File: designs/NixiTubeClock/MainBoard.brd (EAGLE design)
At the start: 94 x 45 mm, 18 parts, among them IC1 LD117ADT-TR, J1 S2B-PH-SM4, J2 S2B-PH-SM4, J3 S2B-PH-SM4, J4 S2B-PH-SM4, J5 S2B-PH-SM4, J6 S2B-PH-SM4, J7 S2B-PH-SM4

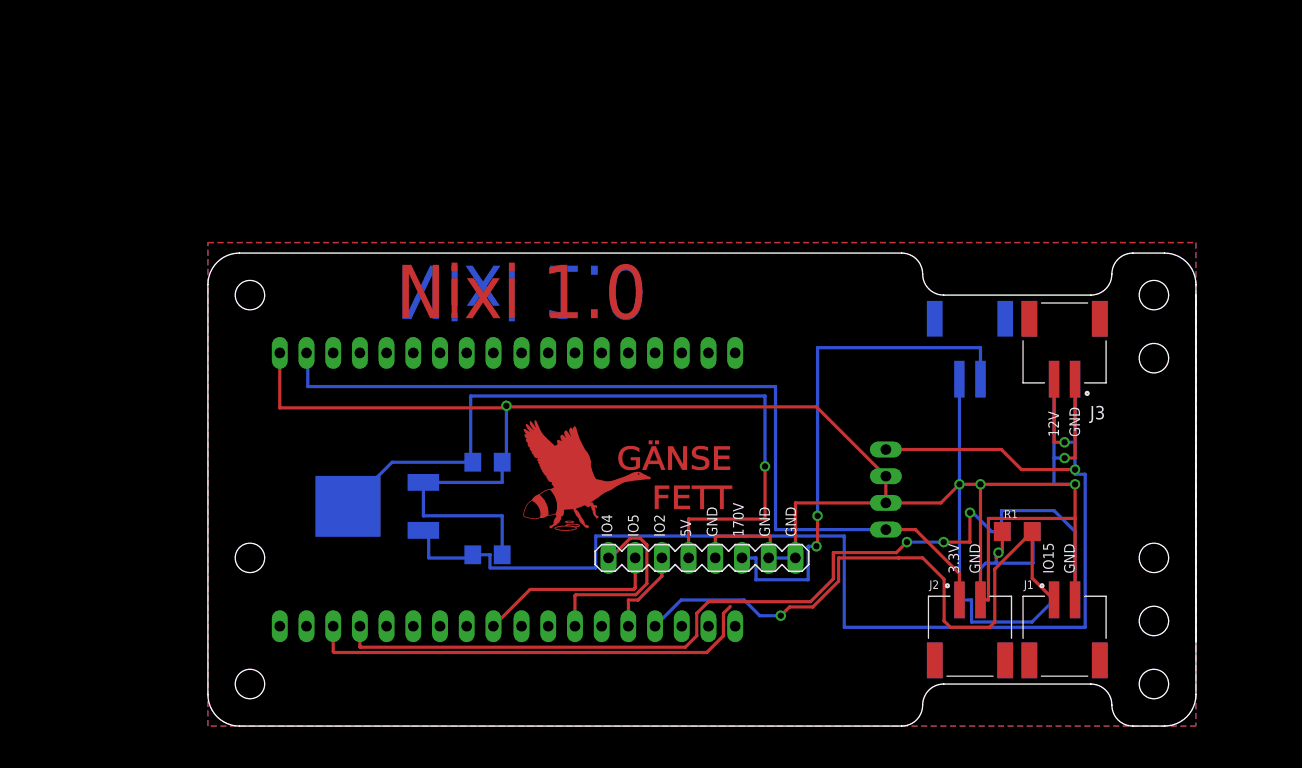
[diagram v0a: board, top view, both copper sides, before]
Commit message: started work on mainboard
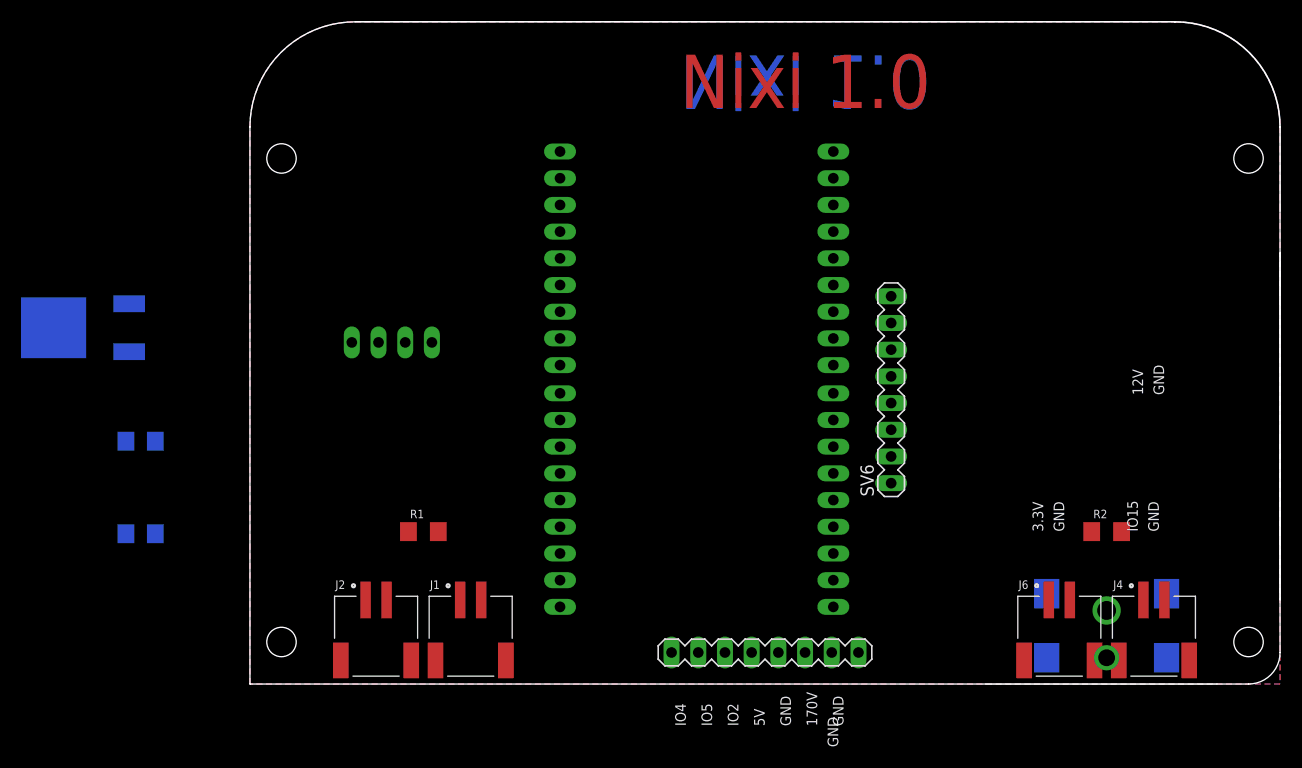
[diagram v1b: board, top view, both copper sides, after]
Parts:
- removed J3, J7: S2B-PH-SM4, CommonParts:JST_S2B-PH-SM4-TB(LF)(SN)
- added SV6: (no value), CommonParts:MA08-1
- J5: value S2B-PH-SM4 -> PJ-002AH-SMT-TR; device CommonParts:JST_S2B-PH-SM4-TB(LF)(SN) -> CommonParts:PJ-002AH-SMT-TR
- moved J1 56.5 mm to (21.0, 8.00)
- moved J2 56.5 mm to (12.0, 8.00)
- moved R1 56.5 mm to (16.5, 14.5)
- moved JP1 49.0 mm to (13.5, 32.5), turned to 180 degrees
- moved SV5 44.2 mm to (55.5, 17.5), turned to 90 degrees
- moved SV4 40.1 mm to (55.5, 40.5), turned to 90 degrees
- moved C1 33.1 mm to (-10.4, 14.3)
- moved C2 33.1 mm to (-10.4, 23.1)
- moved IC1 32.8 mm to (-16.3, 33.9)
- moved J5 31.5 mm to (77.0, -2.50), turned to 90 degrees
- moved SV2 18.8 mm to (29.5, 40.5), turned to 270 degrees
- moved SV3 15.4 mm to (29.5, 17.5), turned to 270 degrees
- moved SV1 10.8 mm to (49.0, 3.00)
- moved J4 8.50 mm to (86.0, 8.00), flipped to the top
- moved J6 8.50 mm to (77.0, 8.00), flipped to the top
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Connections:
- net 12V: no longer J3.2, J5.2
- net 170V: no longer J7.2
- net GND: no longer J3.1, J5.1, J7.1
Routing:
- net GND: track 235.6 -> 0.00 mm, vias 5 -> 0
- net 12V: track 130.2 -> 0.00 mm, vias 2 -> 0
- net 3.3V: track 99.2 -> 0.00 mm, vias 1 -> 0
- net RXD0: track 89.9 -> 0.00 mm, vias 3 -> 0
- net 5V: track 70.6 -> 0.00 mm, vias 1 -> 0
- net IO15: track 60.3 -> 0.00 mm, vias 1 -> 0
- net 170V: track 49.8 -> 0.00 mm, vias 2 -> 0
- net TXD0: track 43.3 -> 0.00 mm
- net IO4: track 18.6 -> 0.00 mm
- net IO5: track 17.9 -> 0.00 mm
- net IO2: track 8.36 -> 0.00 mm
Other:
- board size 94 x 45 mm -> 98 x 63 mm
